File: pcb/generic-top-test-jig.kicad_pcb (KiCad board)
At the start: 2 copper layers, 45 x 39.2 mm, 13 parts, among them P1 CONN_01X16, U1 74HC4051, U2 74HC4067, U3 74HC4067, U4 74HC4067, U5 74HC4067

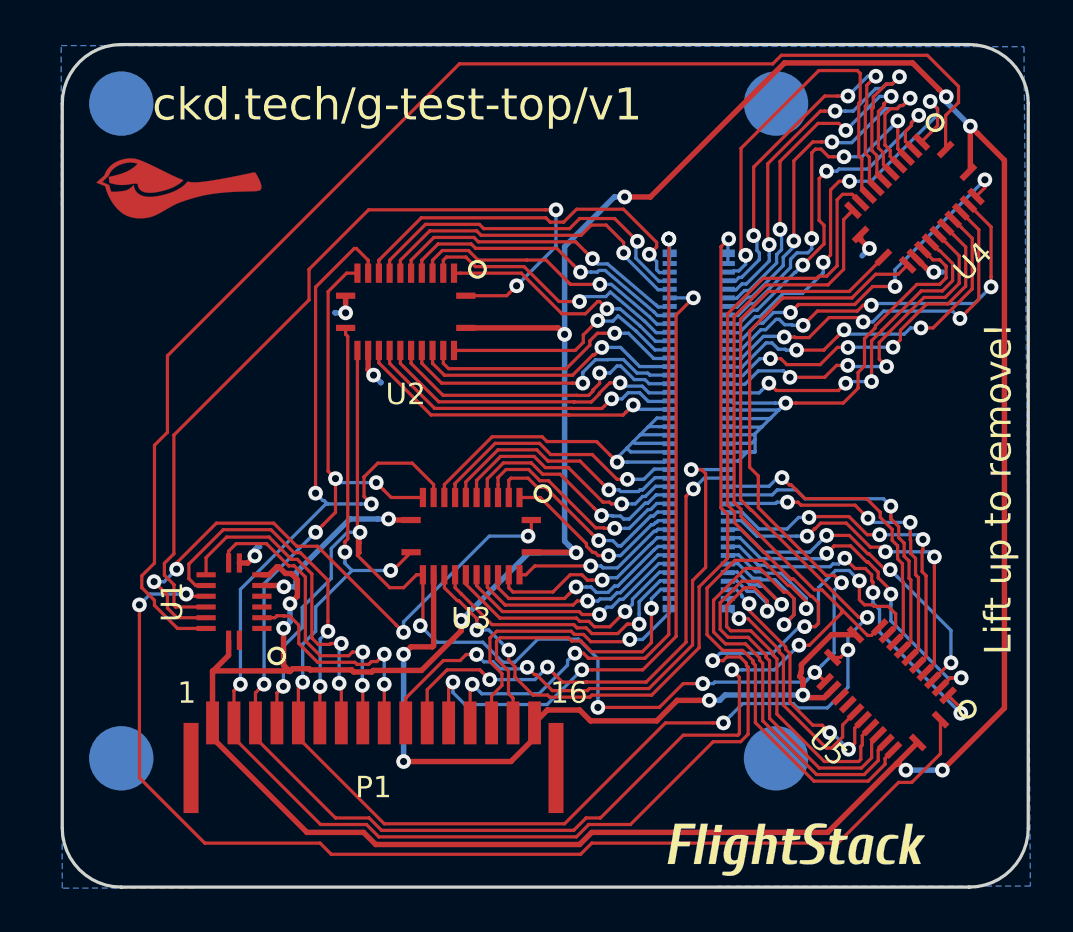
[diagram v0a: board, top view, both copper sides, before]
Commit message: Gerbers for v1 of the test jig.
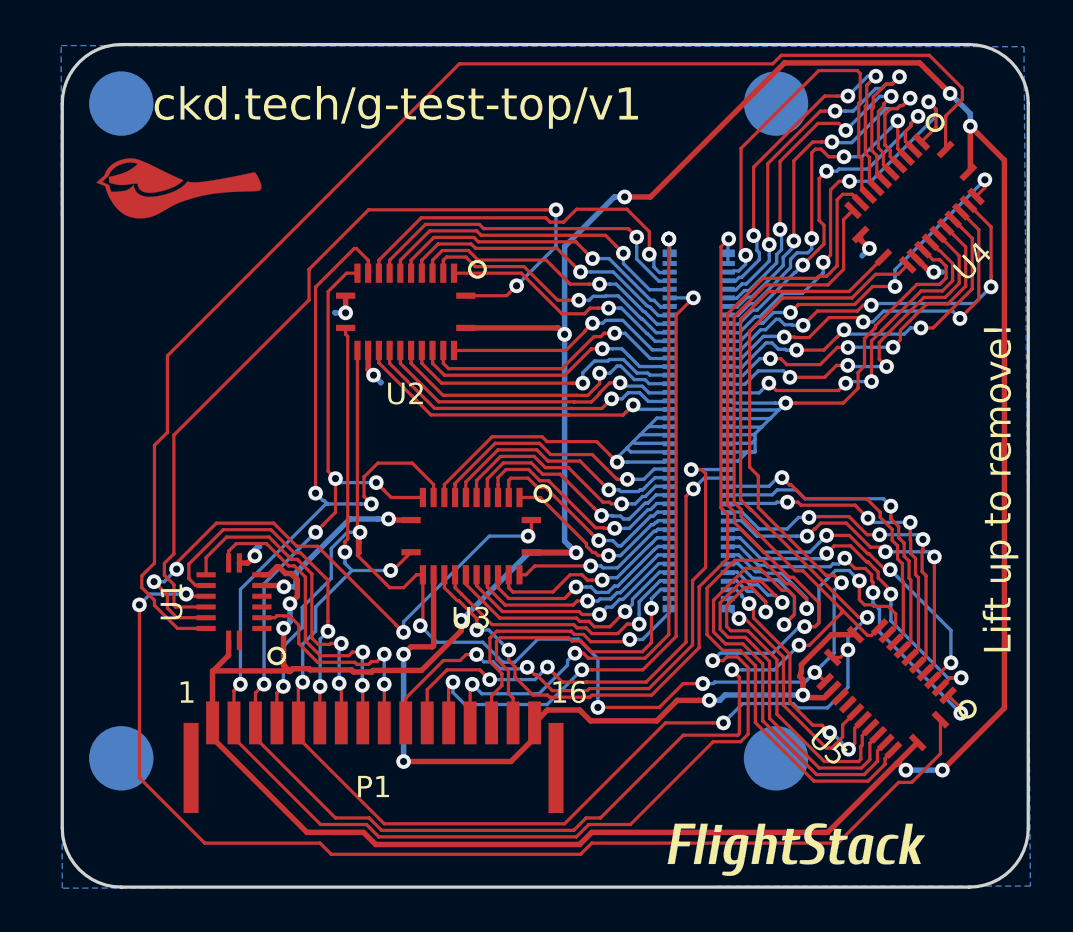
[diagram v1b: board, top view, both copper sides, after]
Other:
- net class Default: clearance 0.1524 -> 0.14986
- net class Power: clearance 0.1524 -> 0.14986
- rule trace_clearance: 0.1524 -> 0.14986
